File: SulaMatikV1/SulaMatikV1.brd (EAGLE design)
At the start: 48.3 x 61 mm, 32 parts, among them IC1 REG1117, Q1 2N3904, Q3 2N3904

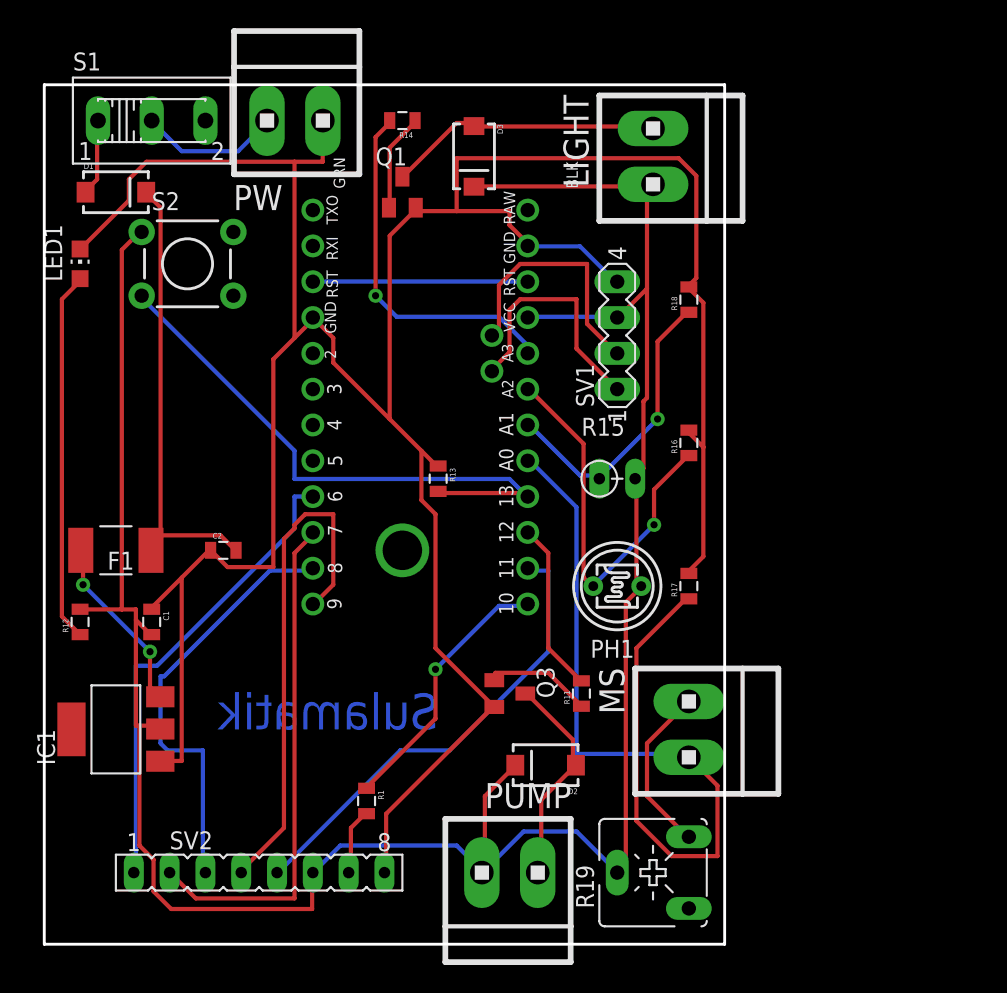
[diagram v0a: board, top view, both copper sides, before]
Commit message: sula5110
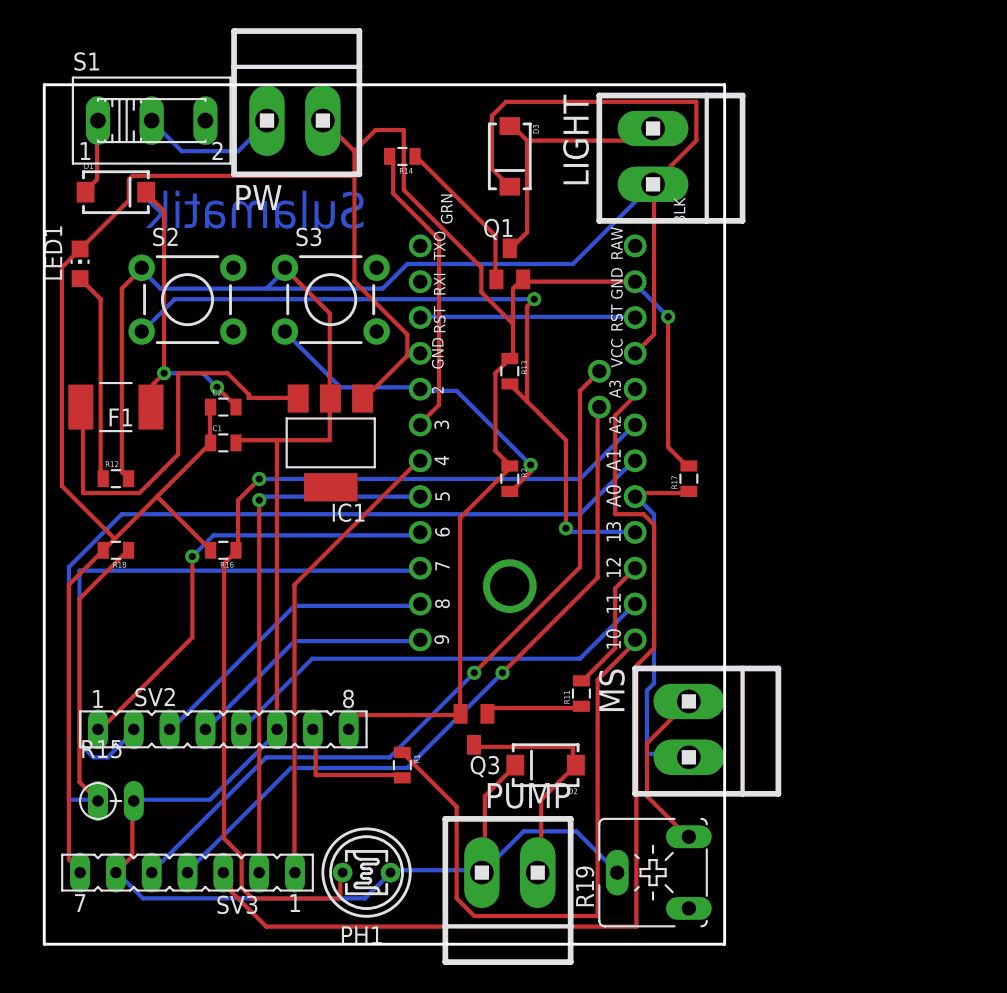
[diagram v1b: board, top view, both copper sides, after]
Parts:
- removed SV1: (no value), con-lstb:MA04-1
- added R2: 10k, SparkFun-Passives:0805
- added S3: SWITCH-MOMENTARY-2PTH, SparkFun-Electromechanical:TACTILE-PTH
- added SV3: (no value), con-lsta:FE07
- moved R18 44.4 mm to (5.08, 27.9), turned to 180 degrees
- moved R15 42.3 mm to (5.08, 10.2)
- moved R16 33.9 mm to (12.7, 27.9), turned to 180 degrees
- moved PH1 27.0 mm to (22.9, 5.08)
- moved IC1 25.4 mm to (20.3, 35.6), turned to 180 degrees
- moved C1 13.7 mm to (12.7, 35.6), turned to 0 degrees
- moved R12 10.5 mm to (5.08, 33.0), turned to 0 degrees
- moved SV2 10.5 mm to (12.7, 15.2)
- moved C2 10.2 mm to (12.7, 38.1)
- moved F1 10.2 mm to (5.08, 38.1)
- moved Q1 9.16 mm to (33.0, 48.3)
- moved R13 9.16 mm to (33.0, 40.6)
- moved JP7 8.03 mm to (26.7, 21.6)
- moved JP2 8.03 mm to (39.4, 38.1)
- moved JP6 8.03 mm to (41.9, 49.5)
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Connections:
- net A3: now also SV3.3; no longer R14.2
- net A4: now also SV3.4; no longer SV1.1
- net A5: now also SV3.5; no longer SV1.2
- net D2: now also R2.2, S3.3
- net D3: now also R14.2
- net D4: now also SV3.1
- net D5: now also SV3.2
- net GND: now also R2.1, SV3.7; no longer SV1.4
- net VCC: now also S3.1, SV3.6; no longer SV1.3
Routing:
- net A1: track 21.2 -> 81.7 mm, vias 1 -> 0
- net A3: track 25.6 -> 72.9 mm, vias 1 -> 0
- net A2: track 28.0 -> 68.0 mm
- net D5: track 0.00 -> 37.9 mm, vias 0 -> 1
- net A0: track 62.5 -> 26.2 mm
- net A5: track 17.9 -> 53.8 mm, vias 0 -> 1
- net D4: track 0.00 -> 33.0 mm
- net A4: track 17.5 -> 49.9 mm, vias 0 -> 1
- net VCC: track 176.2 -> 205.0 mm
- net D10: track 19.0 -> 43.2 mm, vias 1 -> 0
- net D2: track 0.00 -> 23.9 mm, vias 0 -> 1
- net D3: track 0.00 -> 21.0 mm
- net D9: track 36.3 -> 17.9 mm
- net N$1: track 12.7 -> 29.2 mm, vias 2 -> 0
- net GND: track 215.0 -> 199.0 mm, vias 0 -> 1
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
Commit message: sula1
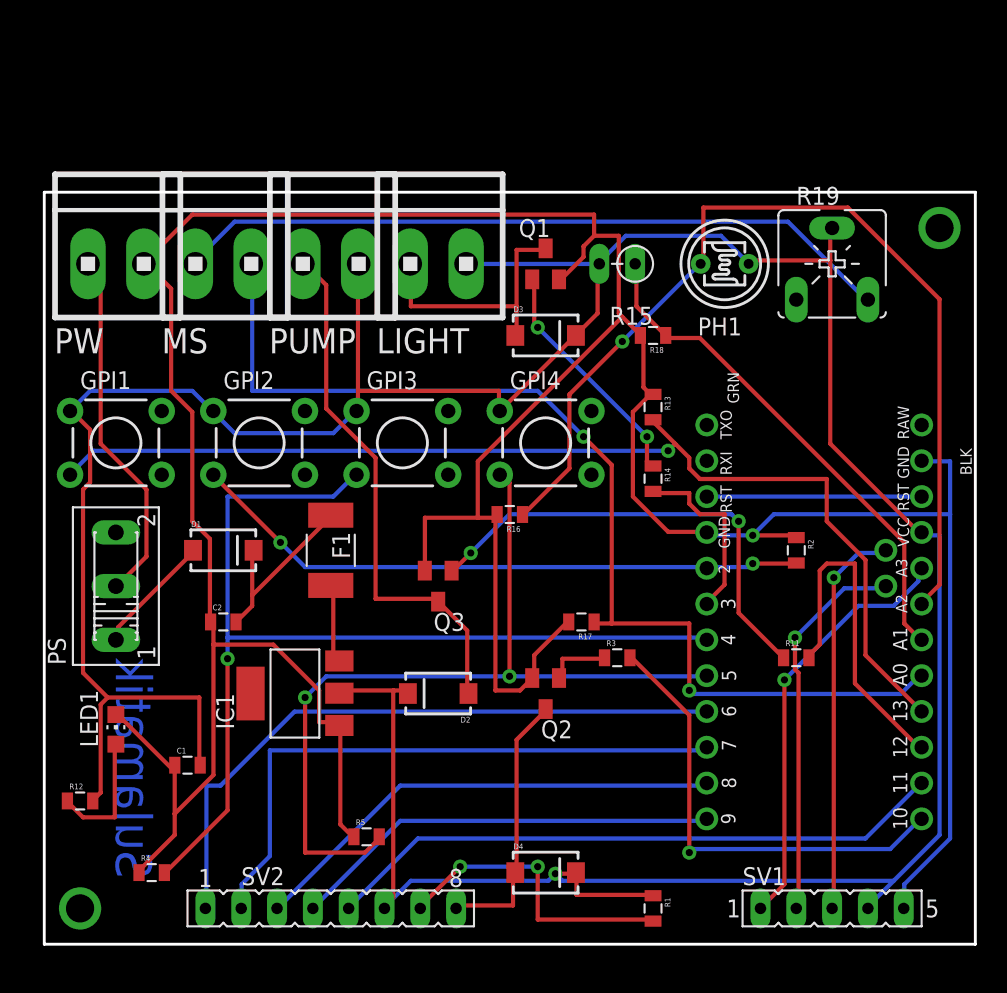
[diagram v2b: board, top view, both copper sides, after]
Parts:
- removed S1: (no value), switch:255SB
- removed S2, S3: SWITCH-MOMENTARY-2PTH, SparkFun-Electromechanical:TACTILE-PTH
- removed SV3: (no value), con-lsta:FE07
- added D4: (no value), SparkFun-DiscreteSemi:SMA-DIODE
- added GPI1, GPI2, GPI3, GPI4: SWITCH-MOMENTARY-2PTH, SparkFun-Electromechanical:TACTILE-PTH
- added PS: (no value), switch:255SB
- added Q2: 2N5551, semicon-smd-ipc:SOT23
- added R3: 1K, SparkFun-Passives:0805
- added R4, R5: 10k, SparkFun-Passives:0805
- added SV1: (no value), con-lsta:FE05-1
- Q3: value 2N3904 -> 2N5551
- moved R15 52.1 mm to (40.6, 48.3), turned to 180 degrees
- moved PH1 50.1 mm to (48.3, 48.3)
- moved MS 46.7 mm to (12.7, 48.3), turned to 0 degrees
- moved PUMP 45.0 mm to (20.3, 48.3), turned to 0 degrees
- moved R19 45.0 mm to (55.9, 48.3), turned to 0 degrees
- moved R18 41.0 mm to (43.2, 43.2)
- moved LED1 33.1 mm to (5.08, 15.2)
- moved R14 29.0 mm to (43.2, 33.0), turned to 270 degrees
- moved D1 26.5 mm to (12.7, 27.9)
- moved JP2 24.0 mm to (59.7, 25.4)
- moved JP6 24.0 mm to (62.2, 36.8)
- moved JP7 24.0 mm to (47.0, 8.89)
- moved C1 23.0 mm to (10.2, 12.7)
- moved R12 23.0 mm to (2.54, 10.2)
- moved R2 20.9 mm to (53.3, 27.9)
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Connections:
- new net N$7: Q2.1, R3.1
- new net N$8: D4.A, Q2.3, SV2.8
- net A3: now also SV1.1; no longer SV3.3
- net A4: now also SV1.2; no longer SV3.4
- net A5: now also SV1.3; no longer SV3.5
- net D10: now also R3.2; no longer R1.1
- net D2: now also GPI2.3; no longer S3.3
- net D4: now also GPI3.3, R4.2; no longer SV3.1
- net D5: now also GPI4.3, R5.2; no longer SV3.2
- net GND: now also Q2.2, R4.1, R5.1, SV1.5; no longer SV2.8, SV3.7
- net N$13: now also PS.1; no longer S1.1
- net N$2: now also PS.2; no longer S1.2
- net SCK: now also GPI1.3; no longer S2.3
- net VCC: now also D4.C, GPI1.1, GPI2.1, GPI3.1, GPI4.1, R1.1, SV1.4; no longer S2.1, S3.1, SV3.6
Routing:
- net GND: track 199.0 -> 250.0 mm
- net A0: track 26.2 -> 76.7 mm, vias 0 -> 2
- net A1: track 81.7 -> 36.5 mm
- net VCC: track 205.0 -> 248.1 mm, vias 0 -> 1
- net A3: track 72.9 -> 30.3 mm, vias 0 -> 1
- net D4: track 33.0 -> 72.4 mm, vias 0 -> 1
- net N$17: track 12.1 -> 51.3 mm
- net N$6: track 7.09 -> 33.2 mm, vias 0 -> 2
- net A5: track 53.8 -> 28.0 mm
- net SCK: track 53.1 -> 77.7 mm, vias 2 -> 1
- net N$1: track 29.2 -> 5.61 mm
- net A4: track 49.9 -> 27.3 mm
- net D5: track 37.9 -> 60.6 mm, vias 1 -> 2
- net N$5: track 17.4 -> 37.9 mm
- net D2: track 23.9 -> 44.3 mm, vias 1 -> 2
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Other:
- board size 48.3 x 61 mm -> 66 x 53.3 mm
